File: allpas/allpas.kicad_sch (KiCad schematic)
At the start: 7 parts, among them U1 TL072

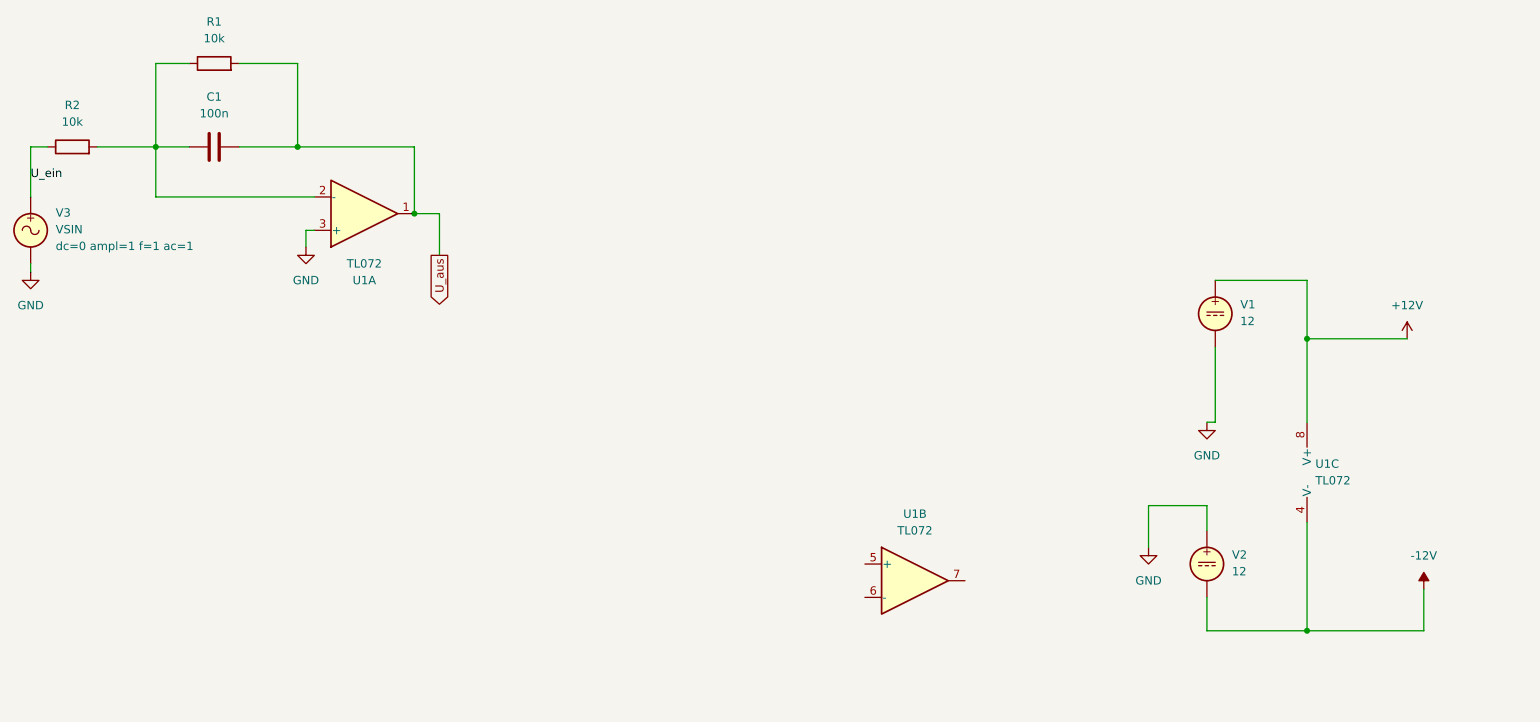
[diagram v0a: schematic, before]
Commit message: adding lagpass and allpass
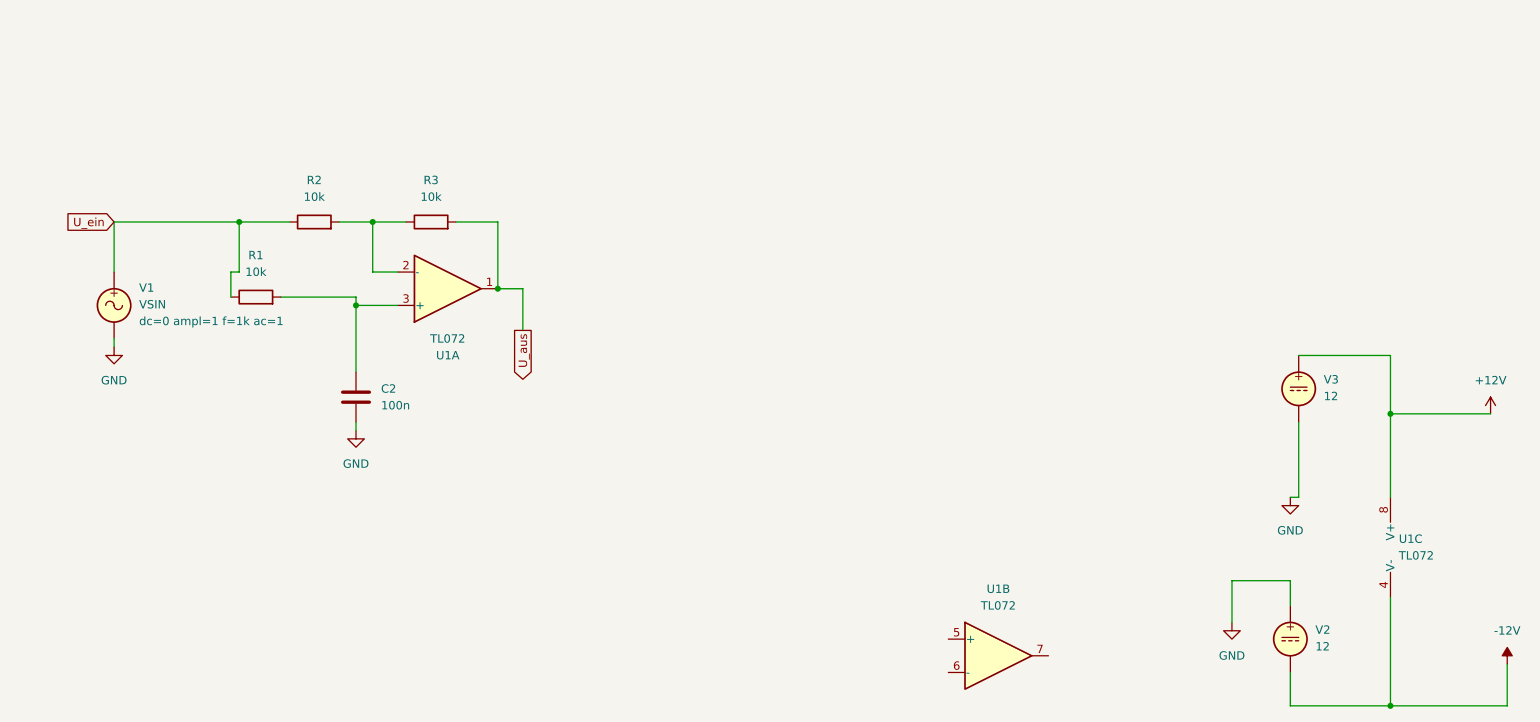
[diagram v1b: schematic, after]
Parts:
- removed C1: 100n, symbol Device:C
- removed V1: 12, symbol Simulation_SPICE:VDC
- removed V3: VSIN, symbol Simulation_SPICE:VSIN
- added C2: 100n, symbol Device:C
- added R3: 10k, symbol Device:R
- added V1: VSIN, symbol Simulation_SPICE:VSIN
- added V3: 12, symbol Simulation_SPICE:VDC
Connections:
- net +12V: now also V3.1
- net GND: now also C2.2, V1.2, V3.2; no longer U1.3 (+)
- net U_aus: now also R3.2; no longer R1.2
- net U_ein: now also R1.1, V1.1
- net at R2.2, U1.2 (-): now also R3.1; no longer R1.1
- new net: C2.1, R1.2, U1.3 (+)
